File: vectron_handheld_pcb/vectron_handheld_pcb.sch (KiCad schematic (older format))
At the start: 18 parts

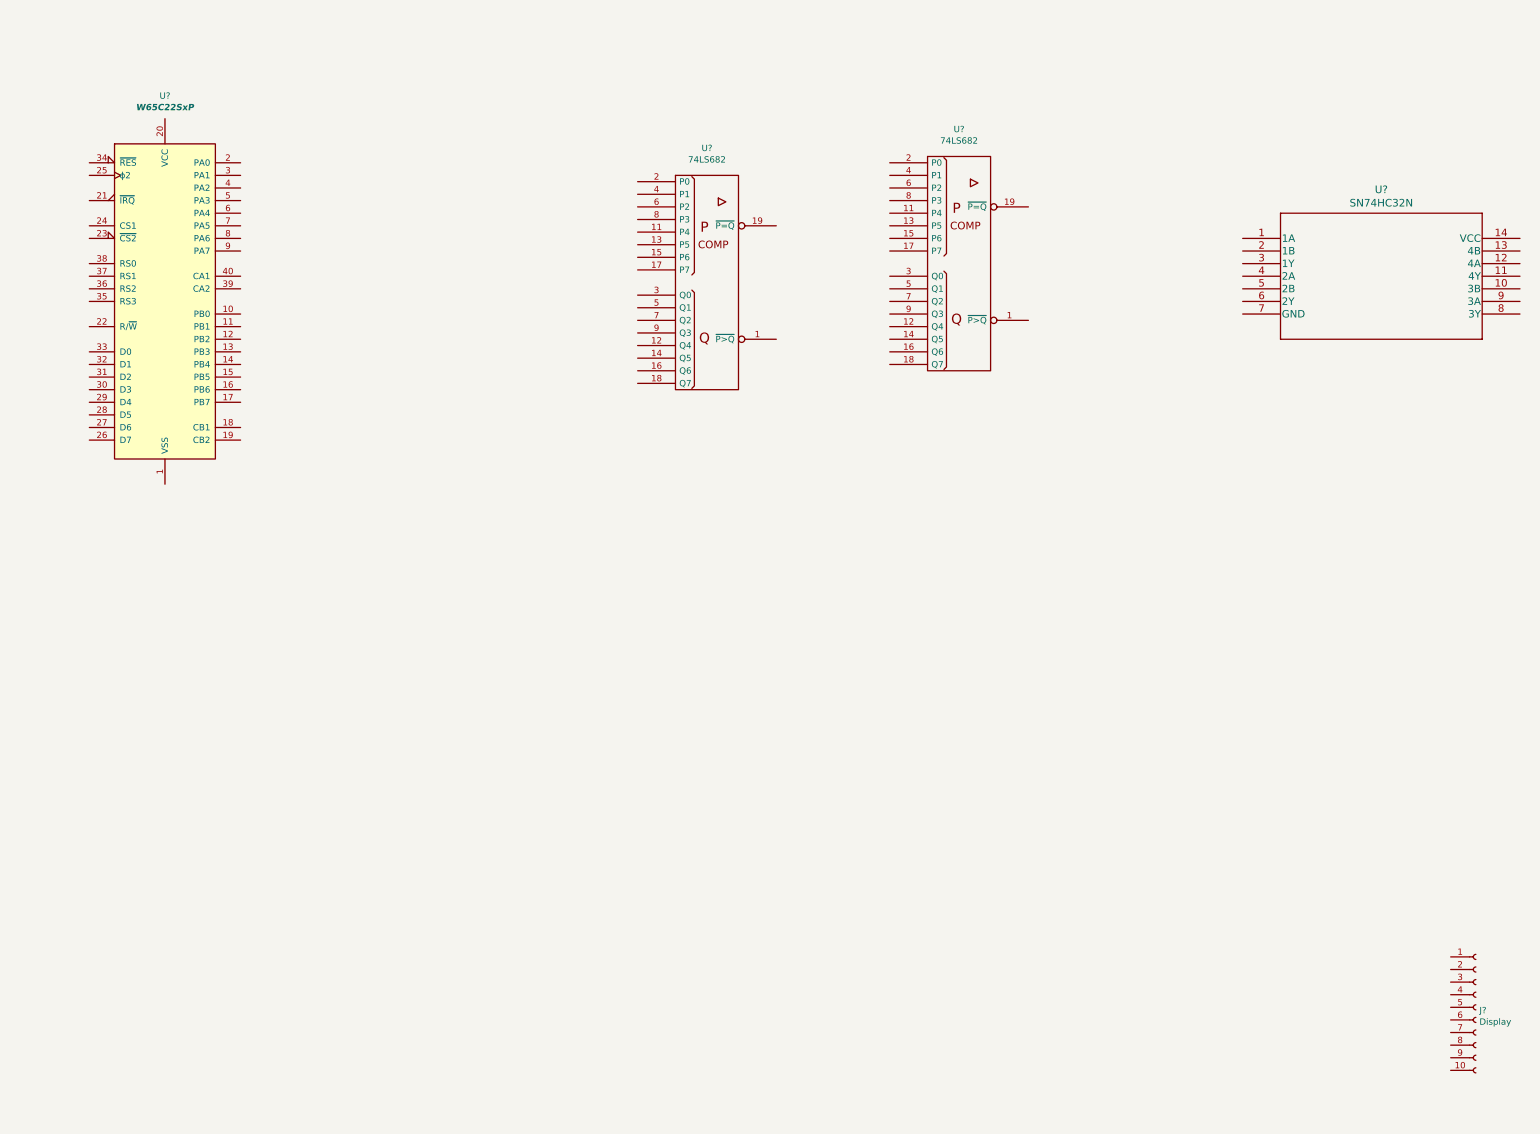
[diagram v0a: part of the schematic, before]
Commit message: Save progress.
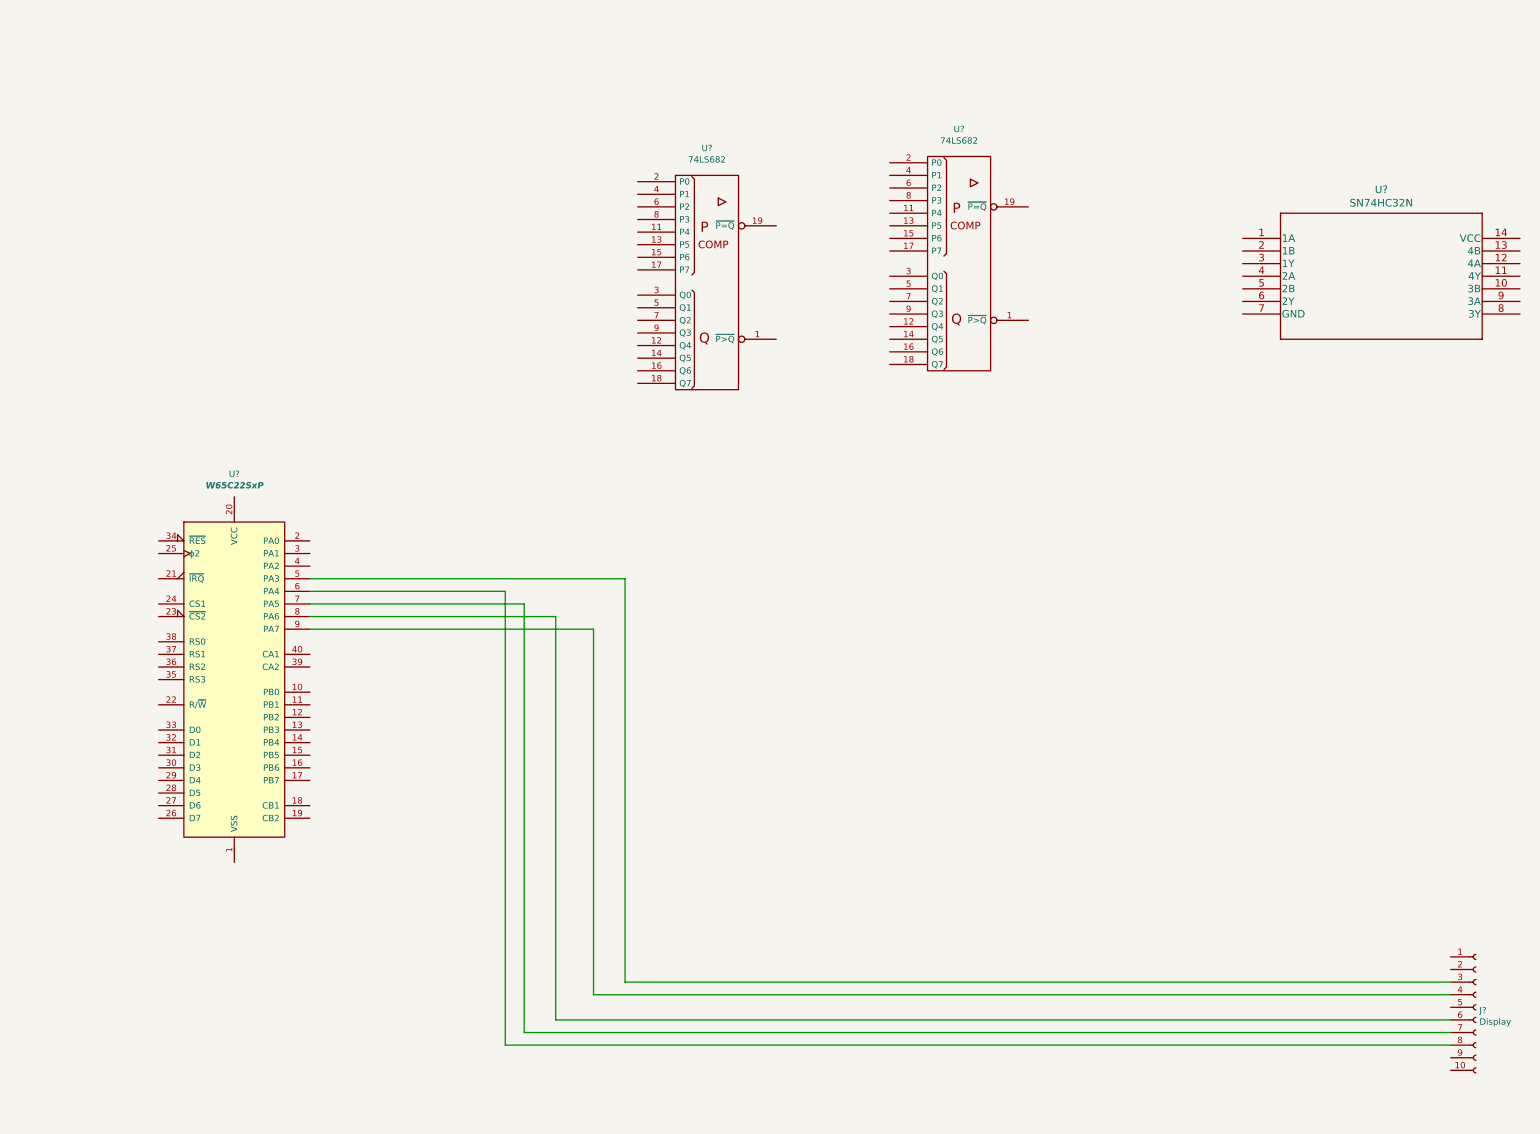
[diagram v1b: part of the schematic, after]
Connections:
- net at U?.5 (PA3): now also J?.3 (Pin_3)
- net at U?.6 (PA4): now also J?.8 (Pin_8)
- net at U?.7 (PA5): now also J?.7 (Pin_7)
- net at U?.8 (PA6): now also J?.6 (Pin_6)
- net at U?.9 (PA7): now also J?.4 (Pin_4)
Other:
- moved on the sheet: U?
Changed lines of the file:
@@
 L 6502:W65C22SxP U?
 U 1 1 5F6BF957
-P 13250 11750
-F 0 "U?" H 13250 13381 50  0000 C CNN
-F 1 "W65C22SxP" H 13250 13290 50  0000 C CIB
-F 2 "" H 13250 11900 50  0001 C CNN
-F 3 "http://www.westerndesigncenter.com/wdc/documentation/w65c22.pdf" H 13250 11900 50  0001 C CNN
-	1    13250 11750
+P 13800 14750
+F 0 "U?" H 13800 16381 50  0000 C CNN
+F 1 "W65C22SxP" H 13800 16290 50  0000 C CIB
+F 2 "" H 13800 14900 50  0001 C CNN
+F 3 "http://www.westerndesigncenter.com/wdc/documentation/w65c22.pdf" H 13800 14900 50  0001 C CNN
+	1    13800 14750
 	1    0    0    -1
 $EndComp
@@
 	1    0    0    -1
 $EndComp
+Wire Wire Line
+	23450 17250 16650 17250
+Wire Wire Line
+	16650 17250 16650 14350
+Wire Wire Line
+	16650 14350 14400 14350
+Wire Wire Line
+	23450 17450 16350 17450
+Wire Wire Line
+	16350 17450 16350 14250
+Wire Wire Line
+	16350 14250 14400 14250
+Wire Wire Line
+	14400 14150 16100 14150
+Wire Wire Line
+	16100 14150 16100 17550
+Wire Wire Line
+	16100 17550 23450 17550
+Wire Wire Line
+	14400 14050 15950 14050
+Wire Wire Line
+	15950 14050 15950 17650
+Wire Wire Line
+	15950 17650 23450 17650
+Wire Wire Line
+	14400 13950 16900 13950
+Wire Wire Line
+	16900 13950 16900 17150
+Wire Wire Line
+	16900 17150 23450 17150
 $EndSCHEMATC
